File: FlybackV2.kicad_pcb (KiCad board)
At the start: 2 copper layers, 183.1 x 109.3 mm, 144 parts, among them J1 Power, J10 ads1256, J11 Coils, J2 Conn_01x02, J3 Conn_01x03, Q6 2N3906, T2 0399-T208, U1 LT8304, U10 LT1634BIS8-2.5, U11 MAX4239, U4 7.68MHz, U5 MAX4239, U6 MAX4239, U7 MAX4239, U8 ADS1256IDBR, U9 MAX4239

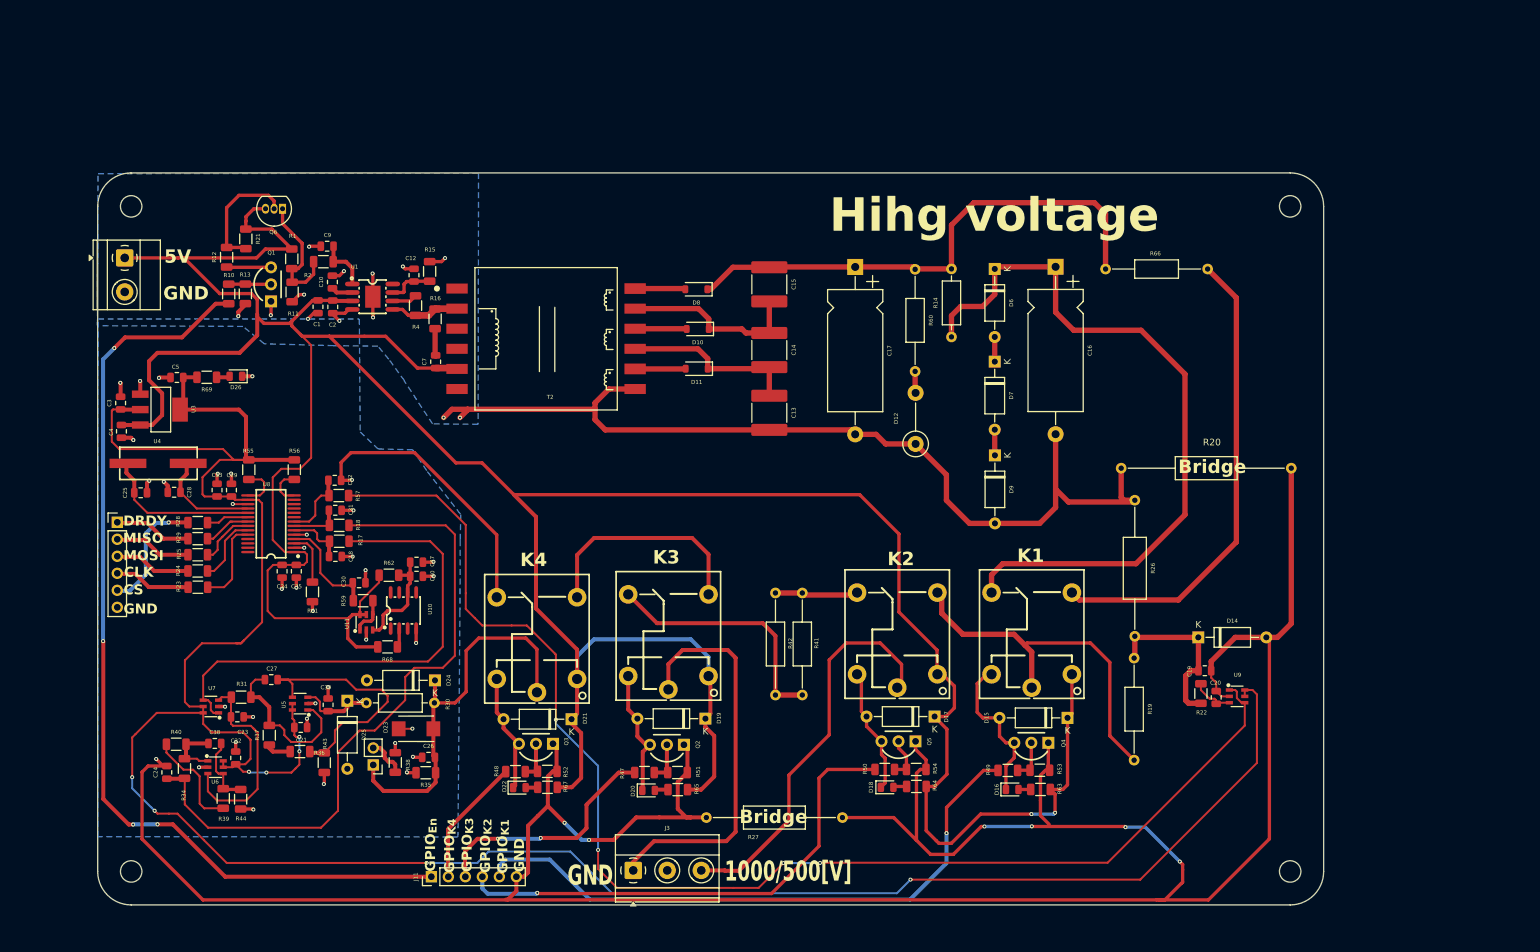
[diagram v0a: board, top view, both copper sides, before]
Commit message: finish v2 version
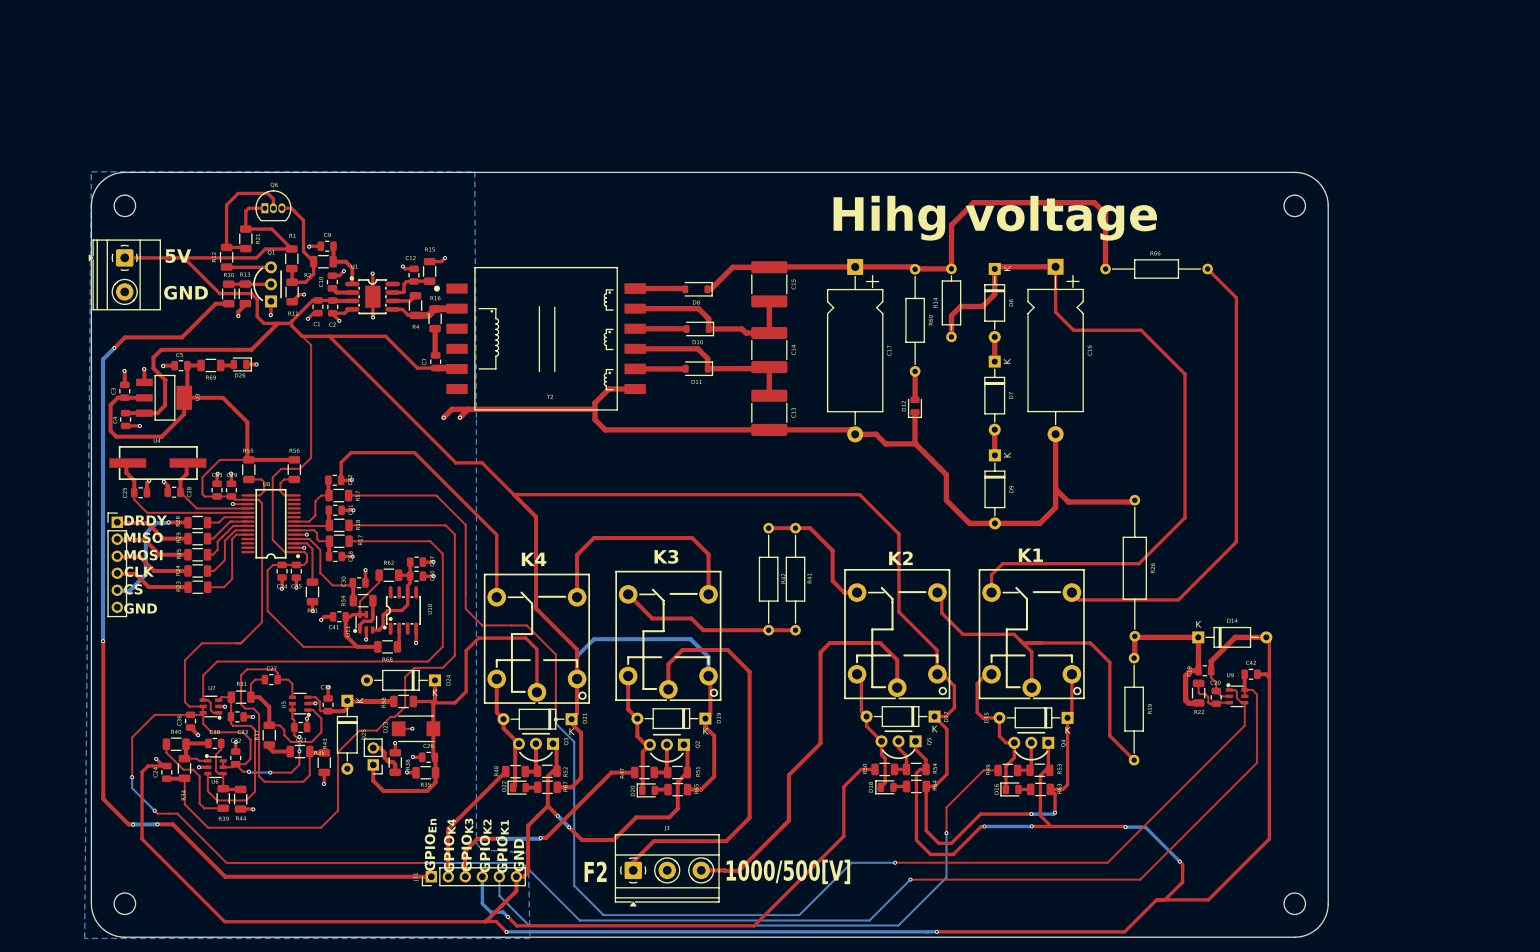
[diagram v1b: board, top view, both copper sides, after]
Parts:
- removed R20: 0, Resistor_THT:R_Axial_DIN0309_L9.0mm_D3.2mm_P25.40mm_Horizontal
- removed R27: 0, Resistor_THT:R_Axial_DIN0309_L9.0mm_D3.2mm_P20.32mm_Horizontal
- removed R30: 100, Resistor_THT:R_Axial_DIN0207_L6.3mm_D2.5mm_P10.16mm_Horizontal
- added C36: 10u, Capacitor_SMD:C_0805_2012Metric, F.Cu at (69.1, 124.3)
- added C41: 10u, Capacitor_SMD:C_0805_2012Metric, F.Cu at (91.3, 108.7)
- added C42: 10u, Capacitor_SMD:C_0805_2012Metric, F.Cu at (227.4, 117.3)
- added R58: 100, Resistor_SMD:R_1206_3216Metric, F.Cu at (100.9, 121.4)
- D12: footprint Resistor_THT:R_Axial_DIN0411_L9.9mm_D3.6mm_P7.62mm_Vertical -> LED_SMD:LED_0805_2012Metric
- moved R41 9.73 mm to (159.4, 110.7)
- moved R42 9.73 mm to (155.4, 110.7)
- moved D12 5.65 mm to (177.2, 77.2)
- moved H3 4.91 mm to (59.3, 151.6)
- moved H2 4.87 mm to (234.0, 151.6)
- moved Q6 2.64 mm to (80.2, 47.7), turned to 0 degrees
- moved D26 1.87 mm to (76.5, 71.0)
- moved C3 1.87 mm to (59.2, 75.0)
- moved C5 1.87 mm to (67.6, 71.2)
- moved C4 1.87 mm to (59.4, 79.3)
- moved R69 1.87 mm to (72.1, 71.2)
- moved U3 1.87 mm to (65.1, 76.0)
- moved H4 0.94 mm to (59.3, 47.3)
- moved H1 0.69 mm to (234.0, 47.3)
- moved R22 0.35 mm to (219.6, 120.1)
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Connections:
- Q6 pad 1: Net-(Q6-E) -> +5V
- Q6 pad 3: +5V -> Net-(Q6-C)
- R1 pad 2: Net-(Q6-E) -> Net-(Q6-C)
- R11 pad 1: Net-(Q6-E) -> Net-(Q6-C)
- R2 pad 2: Net-(Q6-E) -> Net-(Q6-C)
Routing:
- net GND: track 701.0 -> 666.6 mm, vias 56 -> 60
- net Net-(Q6-E): track 19.0 -> 0.00 mm
- net Net-(Q6-C): track 0.00 -> 18.4 mm
- net Net-(R41-Pad1): track 37.4 -> 27.2 mm
- net Net-(D25-K): track 11.8 -> 20.9 mm
- net Net-(R33-Pad3): track 12.5 -> 19.8 mm
- net /ADC2: track 197.6 -> 204.5 mm, vias 4 -> 2
- net Net-(U5-IN-): track 38.7 -> 42.6 mm
- net /GPIO_{K2}: track 74.4 -> 78.0 mm
- net +5V: track 517.0 -> 520.5 mm
- net /In_{pos}: track 58.4 -> 61.6 mm
- net /GPIO_{K1}: track 91.9 -> 94.9 mm
- net Net-(R19-Pad2): track 54.6 -> 57.5 mm
- net /GPIO_{K3}: track 36.1 -> 34.0 mm
- net +3.3_{iso}V: track 380.2 -> 378.3 mm
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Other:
- board size 183.1 x 109.3 mm -> 184.7 x 114.2 mm
- board text added: "F2"
- board text removed: "Bridge"

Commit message: update: init the track of the pcb
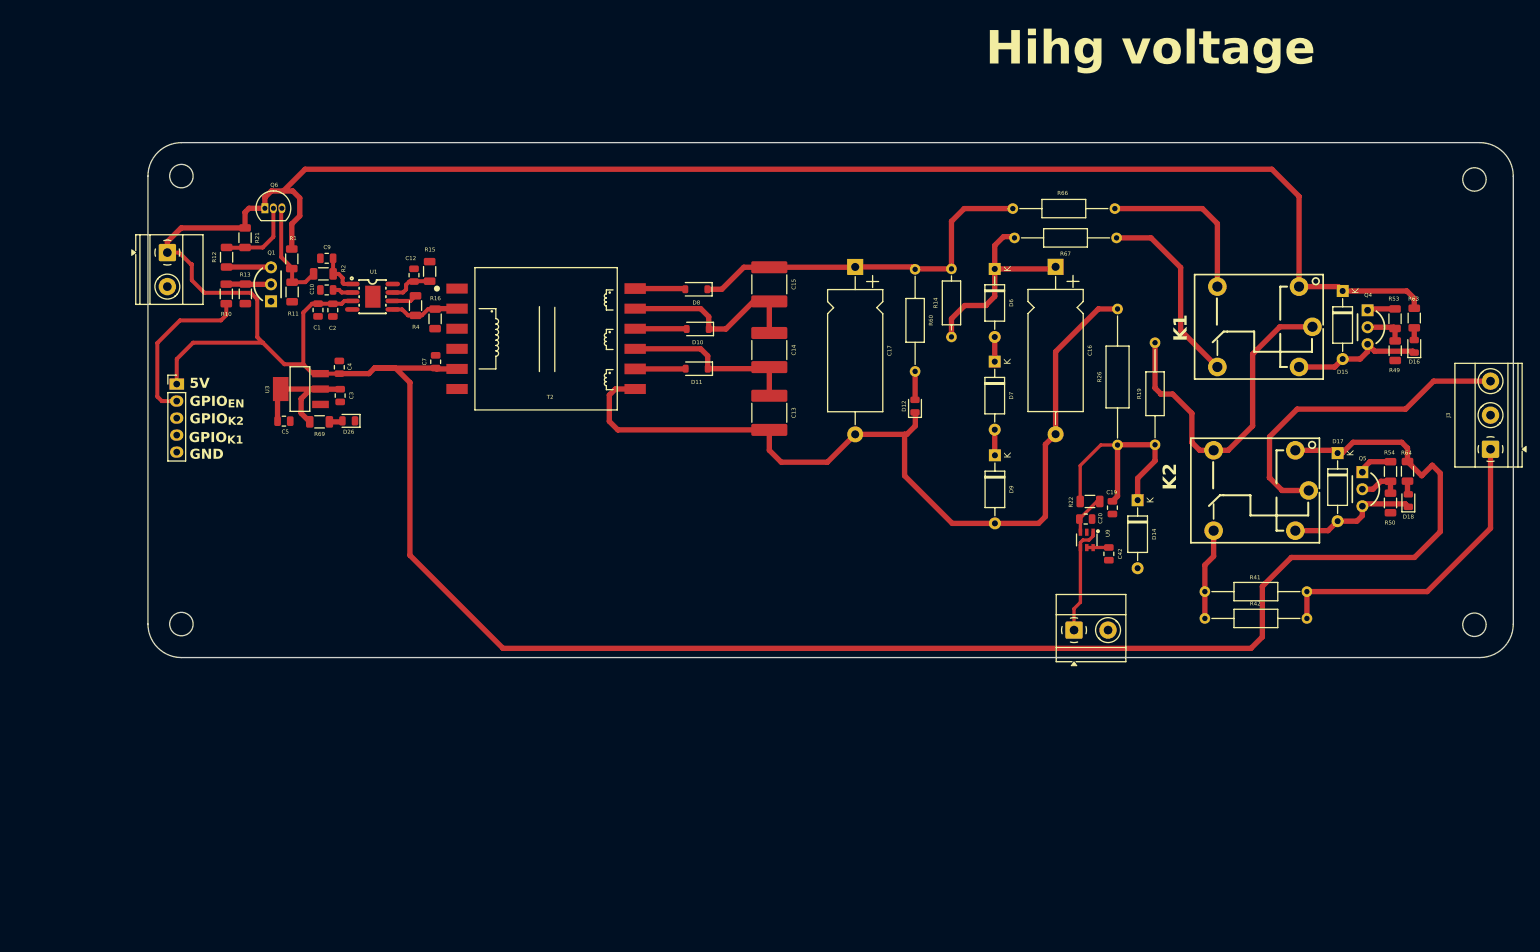
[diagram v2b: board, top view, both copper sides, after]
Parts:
- removed C18, C31, C32: 100nF, Capacitor_SMD:C_0805_2012Metric
- removed C21, C22, C23, C24, C29, C30, C34, C36, C37, C41: 10u, Capacitor_SMD:C_0805_2012Metric
- removed C25, C28: 20pF, Capacitor_SMD:C_0805_2012Metric
- removed C26, C27, C38, C39: 1u, Capacitor_SMD:C_0805_2012Metric
- removed C33, C35, C40: 0.1u, Capacitor_SMD:C_0805_2012Metric
- removed D19, D21: D_Small_Filled, Diode_THT:D_A-405_P10.16mm_Horizontal
- removed D20, D22: LED, LED_SMD:LED_0805_2012Metric
- removed D23: SMBJ5.0CA, JuanDavid_Library:SMB_L4.6-W3.6-LS5.3-BI
- removed D24, D25: D_Zener_Small_Filled, Diode_THT:D_A-405_P10.16mm_Horizontal
- removed J10: ads1256, Connector_PinHeader_2.54mm:PinHeader_1x06_P2.54mm_Vertical
- removed J11: Coils, Connector_PinHeader_2.54mm:PinHeader_1x06_P2.54mm_Vertical
- removed Q2, Q3: ~, JuanDavid_Library:TO-92-3_L4.9-W3.7-P2.54-L
- removed R17, R18, R43, R44, R51, R52, R57, R65: 1K, Resistor_SMD:R_1206_3216Metric
- removed R23, R24, R25, R28, R29, R31, R34, R55, R56, R58, R59: 100, Resistor_SMD:R_1206_3216Metric
- removed R35: 10K, Resistor_SMD:R_1206_3216Metric
- removed R36, R39: 2.2K, Resistor_SMD:R_1206_3216Metric
- removed R37, R40: 6.8K, Resistor_SMD:R_1206_3216Metric
- removed R38: 10, Resistor_SMD:R_1206_3216Metric
- removed R45, R46: ~, JuanDavid_Library:RELAY-TH_SRD-XXVDC-XL-C
- removed R47, R48: 560, Resistor_SMD:R_1206_3216Metric
- removed R61, R68: 0, Resistor_SMD:R_1206_3216Metric
- removed R62: 4, Resistor_SMD:R_1206_3216Metric
- removed U10: LT1634BIS8-2.5, JuanDavid_Library:SO-8_L4.9-W3.9-P1.27-LS5.9-BL
- removed U11, U5, U6, U7: MAX4239, JuanDavid_Library:SOT-23-6_L2.9-W1.6-P0.95-LS2.9-BL
- removed U4: 7.68MHz, JuanDavid_Library:CRYSTAL-SMD_L11.4-W4.7-LS12.4
- removed U8: ADS1256IDBR, JuanDavid_Library:SSOP-28_L10.2-W5.3-P0.65-LS7.8-BL
- added J4: Coils, Connector_PinHeader_2.54mm:PinHeader_1x05_P2.54mm_Vertical, F.Cu at (67.0, 74.0)
- J2: value Conn_01x02 -> Divisor; footprint Connector_PinHeader_2.54mm:PinHeader_1x02_P2.54mm_Vertical -> TerminalBlock_Phoenix:TerminalBlock_Phoenix_MKDS-1,5-2-5.08_1x02_P5.08mm_Horizontal
- R26: value 47M -> 100K
- R67: value 1K -> 2M; footprint Resistor_SMD:R_1206_3216Metric -> Resistor_THT:R_Axial_DIN0207_L6.3mm_D2.5mm_P15.24mm_Horizontal
- moved J3 142.6 mm to (263.2, 83.7), turned to 90 degrees
- moved R67 118.1 mm to (207.3, 52.1), turned to 180 degrees
- moved J2 106.6 mm to (201.0, 110.7), turned to 0 degrees
- moved R63 89.8 mm to (251.8, 64.1), turned to 90 degrees
- moved D16 89.4 mm to (251.8, 68.3), turned to 90 degrees
- moved D18 88.8 mm to (250.9, 91.4), turned to 90 degrees
- moved R64 87.1 mm to (250.8, 87.0), turned to 90 degrees
- moved R53 85.8 mm to (248.9, 64.2), turned to 90 degrees
- moved R50 85.4 mm to (248.3, 91.7), turned to -90 degrees
- moved R49 85.3 mm to (249.0, 69.0), turned to -90 degrees
- moved R54 83.6 mm to (248.3, 87.0), turned to 90 degrees
- moved R42 80.4 mm to (235.8, 109.0), turned to 180 degrees
- moved Q4 79.8 mm to (244.8, 65.5), turned to -90 degrees
- moved Q5 78.8 mm to (244.1, 89.7), turned to -90 degrees
- moved R41 76.6 mm to (235.8, 105.0), turned to 180 degrees
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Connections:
- J2 pad 1: /In_{pos} -> Net-(J2-Pin_1)
- J2 pad 2: Net-(J2-Pin_2) -> GND
- R32 pad 3: 500V -> Net-(R32-Pad3)
- R41 pad 1: Net-(R41-Pad1) -> Net-(J3-Pin_1)
- R42 pad 1: Net-(R41-Pad1) -> Net-(J3-Pin_1)
- R67 pad 1: Net-(D22-A) -> Net-(R32-Pad3)
- R67 pad 2: +5V -> 500V
- U9 pad 1: /ADC2 -> Net-(J2-Pin_1)
- U9 pad 4: /ADC2 -> Net-(J2-Pin_1)
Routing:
- net GND: track 666.6 -> 139.5 mm, vias 60 -> 0
- net +3.3_{iso}V: track 378.3 -> 24.7 mm, vias 8 -> 0
- net /ADC2: track 204.5 -> 0.00 mm, vias 2 -> 0
- net /GPIO_{EN}: track 141.7 -> 24.9 mm, vias 4 -> 0
- net /ADC1: track 101.2 -> 0.00 mm
- net /GPIO_{K1}: track 94.9 -> 0.00 mm, vias 1 -> 0
- net 500V: track 110.4 -> 31.0 mm
- net /GPIO_{K2}: track 78.0 -> 0.00 mm, vias 1 -> 0
- net /ADC0: track 73.6 -> 0.00 mm
- net /In_{pos}: track 61.6 -> 0.00 mm
- net Net-(R32-Pad2): track 71.1 -> 25.7 mm
- net Net-(U5-IN-): track 42.6 -> 0.00 mm
- net /GPIO_{K3}: track 34.0 -> 0.00 mm, vias 2 -> 0
- net Net-(R45-Pad2): track 34.0 -> 0.00 mm
- net +5V: track 520.5 -> 551.1 mm, vias 2 -> 0
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- removed copper zone on B.Cu, net GND
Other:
- board size 184.7 x 114.2 mm -> 203.9 x 76.9 mm
- board text added: "GPIO_{EN}"
- board text removed: "1000/500[V]"
- board text removed: "CLK"
- board text removed: "CS"
- board text removed: "DRDY"
- board text removed: "F2"
- board text removed: "GPIO_{En}"
- board text removed: "GPIO_{K3}"
- board text removed: "GPIO_{K4}"
- board text removed: "K3"
- board text removed: "K4"
- board text removed: "MISO"
- board text removed: "MOSI"

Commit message: finish the route, in revision
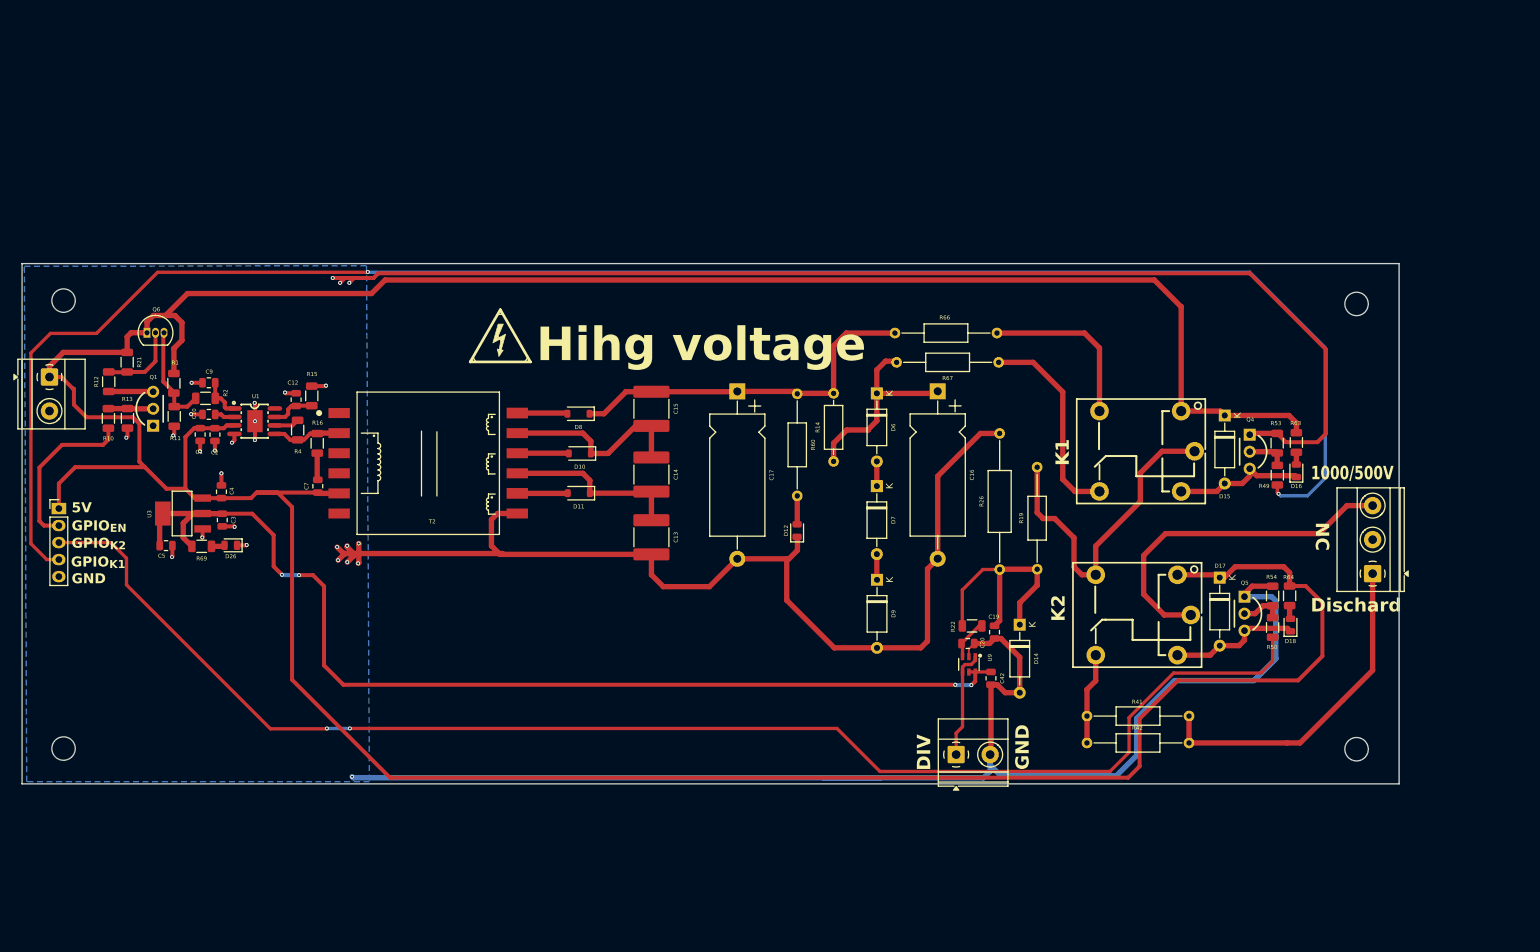
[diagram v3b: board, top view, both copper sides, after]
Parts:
- added REF**: Symbol_HighVoltage_Triangle_6x6mm_Copper, Symbol:Symbol_HighVoltage_Triangle_6x6mm_Copper, F.Cu at (115.3, 66.8)
- moved H1 25.6 mm to (243.2, 62.0)
- moved D10 25.6 mm to (127.2, 84.3)
- moved C10 25.6 mm to (71.8, 78.5)
- moved D17 25.6 mm to (222.8, 102.9)
- moved H2 25.6 mm to (243.2, 128.5)
- moved H3 25.6 mm to (50.1, 128.4)
- moved H4 25.6 mm to (50.1, 61.5)
- moved Q6 25.6 mm to (62.6, 66.3)
- moved R10 25.6 mm to (56.8, 79.1)
- moved R12 25.6 mm to (56.8, 73.6)
- moved R21 25.6 mm to (59.6, 70.7)
- moved C9 25.6 mm to (71.8, 73.8)
- moved D11 25.6 mm to (127.0, 90.2)
- moved D26 25.6 mm to (75.1, 98.0)
- moved J2 25.6 mm to (183.4, 129.3)
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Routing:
- net GND: track 139.5 -> 585.8 mm, vias 0 -> 27
- net /GPIO_{K1}: track 0.00 -> 265.7 mm, vias 0 -> 2
- net /GPIO_{K2}: track 0.00 -> 211.3 mm, vias 0 -> 2
- net +3.3_{iso}V: track 24.7 -> 159.0 mm, vias 0 -> 4
- net Net-(C7-Pad2): track 0.00 -> 4.02 mm
- net Net-(J3-Pin_1): track 47.2 -> 50.4 mm
- net Net-(J3-Pin_3): track 49.3 -> 51.4 mm
- net Net-(R32-Pad3): track 28.5 -> 30.7 mm
- net +5V: track 551.1 -> 552.6 mm
- net Net-(R19-Pad2): track 50.6 -> 49.4 mm
- added copper zone on B.Cu, net GND
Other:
- board size 203.9 x 76.9 mm -> 205.7 x 77.7 mm
- board text added: "1000/500V"
- board text added: "DIV"
- board text added: "Dischard"
- board text added: "NC"
